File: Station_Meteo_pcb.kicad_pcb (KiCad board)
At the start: 2 copper layers, 107 x 64 mm, 123 parts, among them J1 ZX-FPC-FWSX0.5PH224, J10 DZ254S-11-02-48, J11 DZ254S-11-02-48, J2 UC18-0B06F68011, J3 BH127VS-14P-H49, J4 DZ254S-11-02-48, J5 DZ254S-11-02-48, J6 DZ254S-11-02-48, J8 DZ254S-11-02-48, J9 DZ254S-11-02-48, Q1 AO3400A, Q2 AO3400A, Q3 AO3401A, Q5 FS8205A, Q6 AO3401A, Q7 AO3401A, Q8 AO3401A, Q9 AO3400A, U1 BME280, U2 STM32L476RGTx, U3 TP4056-42-ESOP8, U4 TPS63802DLAR, U5 DW01A, Y2 Crystal

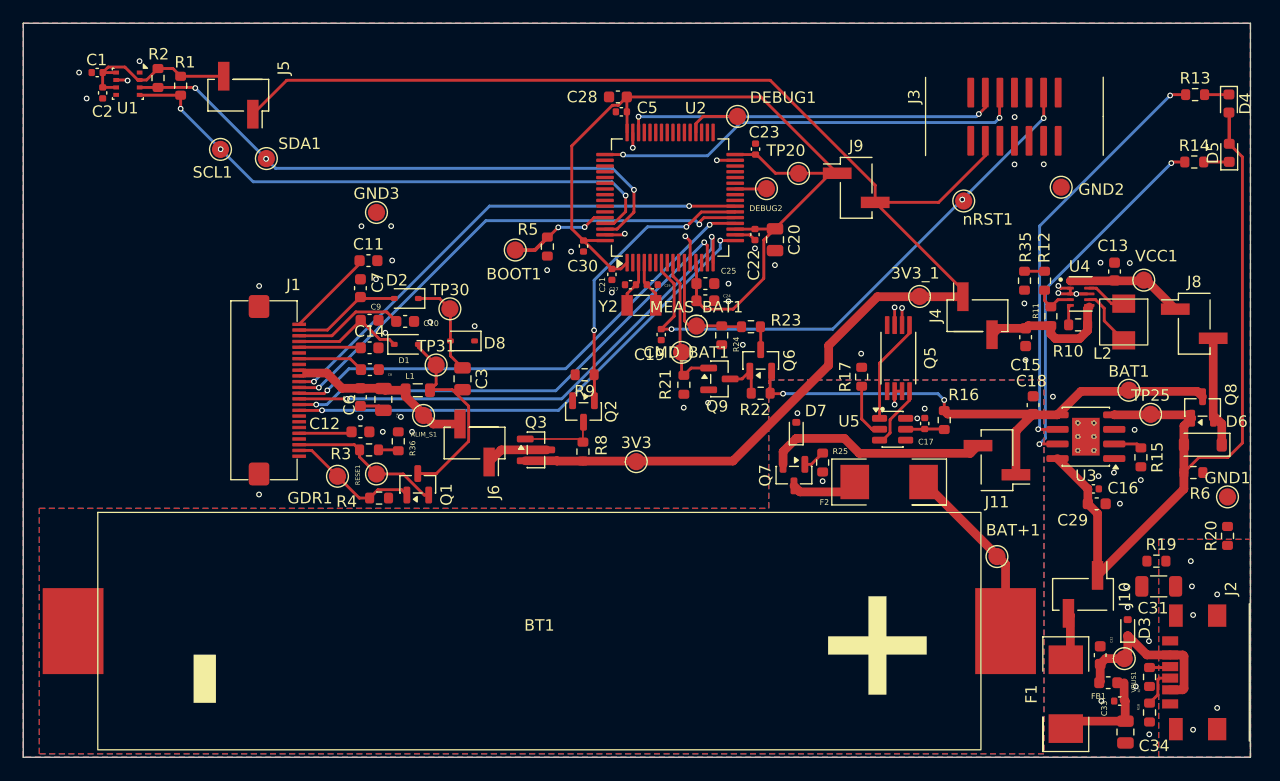
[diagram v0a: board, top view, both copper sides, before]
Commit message: Suite DRC
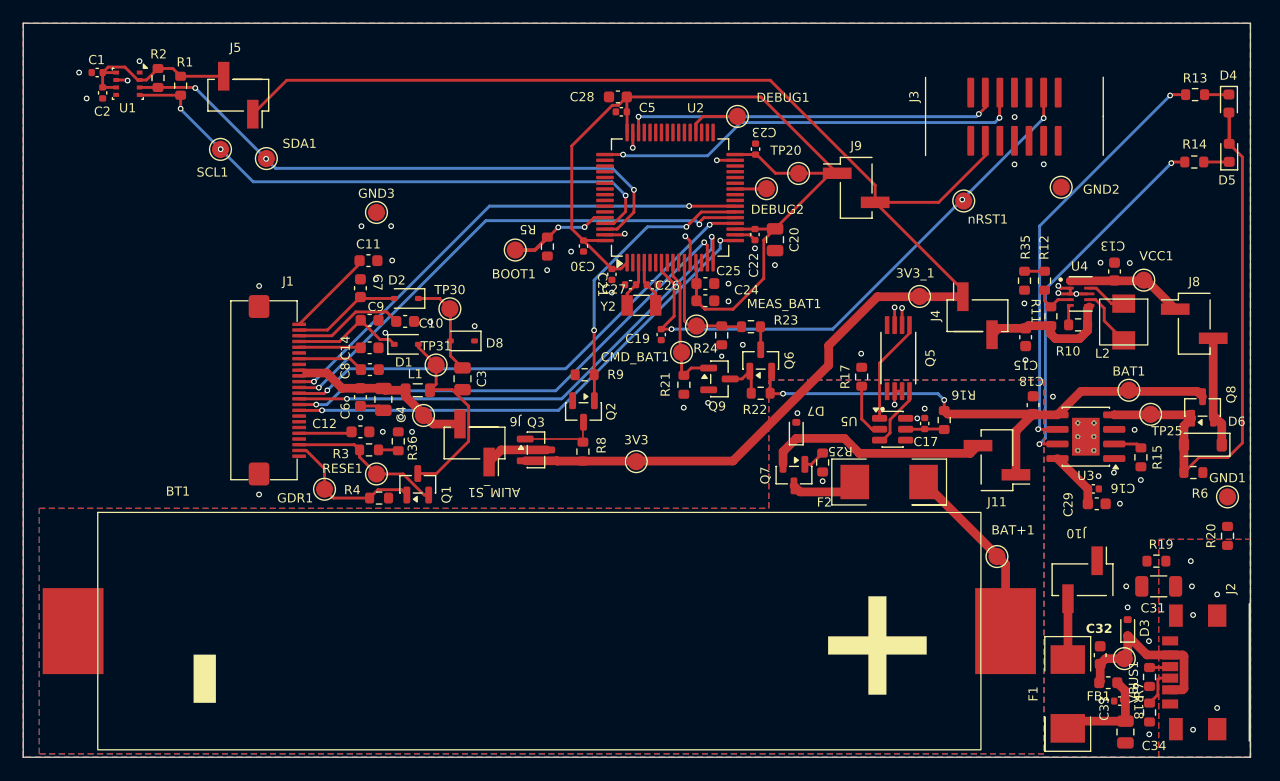
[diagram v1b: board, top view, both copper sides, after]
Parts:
- J1: footprint Composants_Perso:Connector_24P_epaper -> Composants_Perso:Connector_1x24_epaper
- moved GDR1 1.60 mm to (126.3, 86.6)
- moved J10 1.28 mm to (192.4, 94.5)
- moved F1 0.17 mm to (191.1, 104.5)
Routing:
- net VBUS: track 73.8 -> 55.1 mm
- net Net-(J10-Pin_2): track 4.12 -> 5.31 mm
- net GDR: track 11.6 -> 12.7 mm
- net GND: vias 56 -> 57
